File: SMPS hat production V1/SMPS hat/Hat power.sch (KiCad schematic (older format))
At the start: 30 parts, among them Q1 Si4804, Q2 Si4435, U1 LTC4352, U3 LM2576HVS-5, U6 INA219

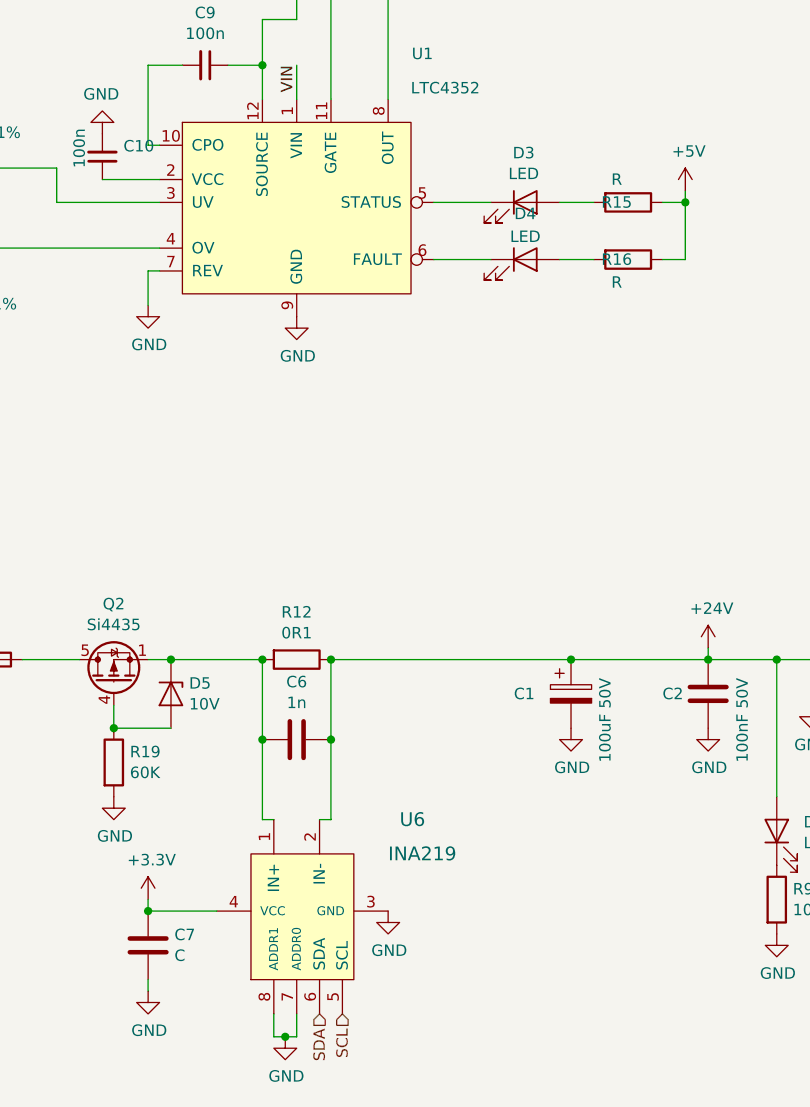
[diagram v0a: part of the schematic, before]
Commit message: sync
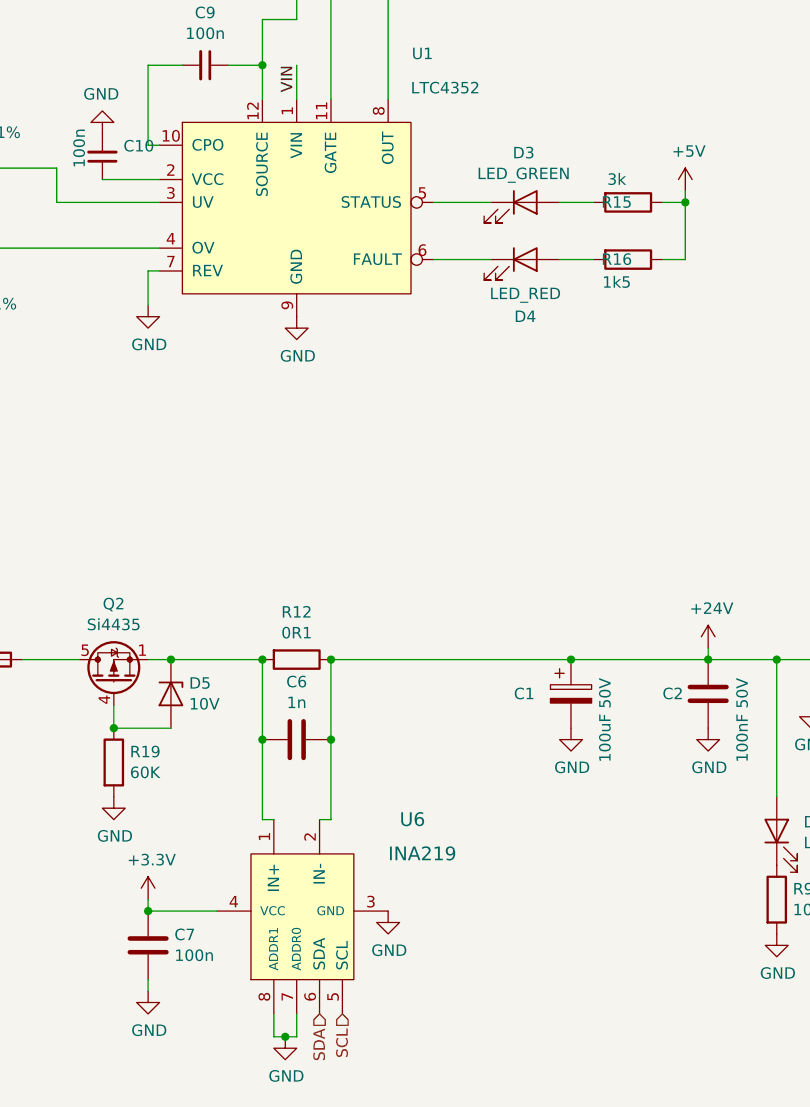
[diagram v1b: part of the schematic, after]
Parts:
- C7: value C -> 100n
- D3: value LED -> LED_GREEN
- D4: value LED -> LED_RED
- R15: value R -> 3k
- R16: value R -> 1k5
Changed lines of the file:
@@
 P 2250 6100
 F 0 "C7" H 2365 6146 50  0000 L CNN
-F 1 "C" H 2365 6055 50  0000 L CNN
+F 1 "100n" H 2365 6055 50  0000 L CNN
 F 2 "Capacitor_SMD:C_0603_1608Metric_Pad1.05x0.95mm_HandSolder" H 2288 5950 50  0001 C CNN
 F 3 "~" H 2250 6100 50  0001 C CNN
@@
 U 1 1 5D4B0215
 P 3900 3100
-F 0 "D4" H 3900 3300 50  0000 C CNN
-F 1 "LED" H 3900 3200 50  0000 C CNN
+F 0 "D4" H 3900 2850 50  0000 C CNN
+F 1 "LED_RED" H 3900 2950 50  0000 C CNN
 F 2 "LED_SMD:LED_0805_2012Metric_Pad1.15x1.40mm_HandSolder" H 3900 3100 50  0001 C CNN
 F 3 "~" H 3900 3100 50  0001 C CNN
@@
 P 3900 2850
 F 0 "D3" H 3893 3066 50  0000 C CNN
-F 1 "LED" H 3893 2975 50  0000 C CNN
+F 1 "LED_GREEN" H 3893 2975 50  0000 C CNN
 F 2 "LED_SMD:LED_0805_2012Metric_Pad1.15x1.40mm_HandSolder" H 3900 2850 50  0001 C CNN
 F 3 "~" H 3900 2850 50  0001 C CNN
@@
 P 4350 3100
 F 0 "R16" V 4350 3050 50  0000 C CNN
-F 1 "R" V 4450 3050 50  0000 C CNN
+F 1 "1k5" V 4450 3050 50  0000 C CNN
 F 2 "Resistor_SMD:R_0805_2012Metric_Pad1.15x1.40mm_HandSolder" V 4280 3100 50  0001 C CNN
 F 3 "~" H 4350 3100 50  0001 C CNN
@@
 P 4350 2850
 F 0 "R15" V 4350 2800 50  0000 C CNN
-F 1 "R" V 4250 2800 50  0000 C CNN
+F 1 "3k" V 4250 2800 50  0000 C CNN
 F 2 "Resistor_SMD:R_0805_2012Metric_Pad1.15x1.40mm_HandSolder" V 4280 2850 50  0001 C CNN
 F 3 "~" H 4350 2850 50  0001 C CNN
